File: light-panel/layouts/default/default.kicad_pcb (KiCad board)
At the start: 2 copper layers, 150 x 29.7 mm, 70 parts

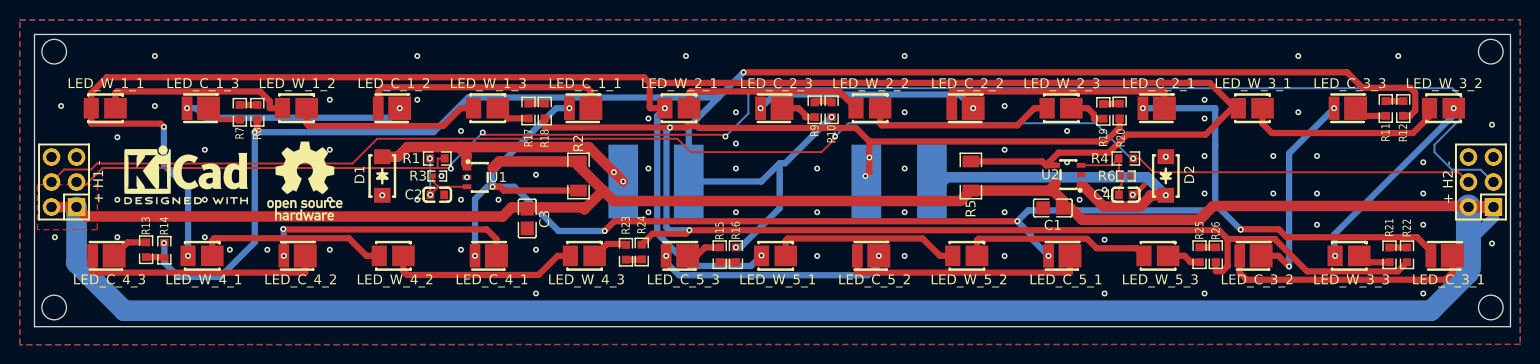
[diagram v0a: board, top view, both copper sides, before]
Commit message: panel router
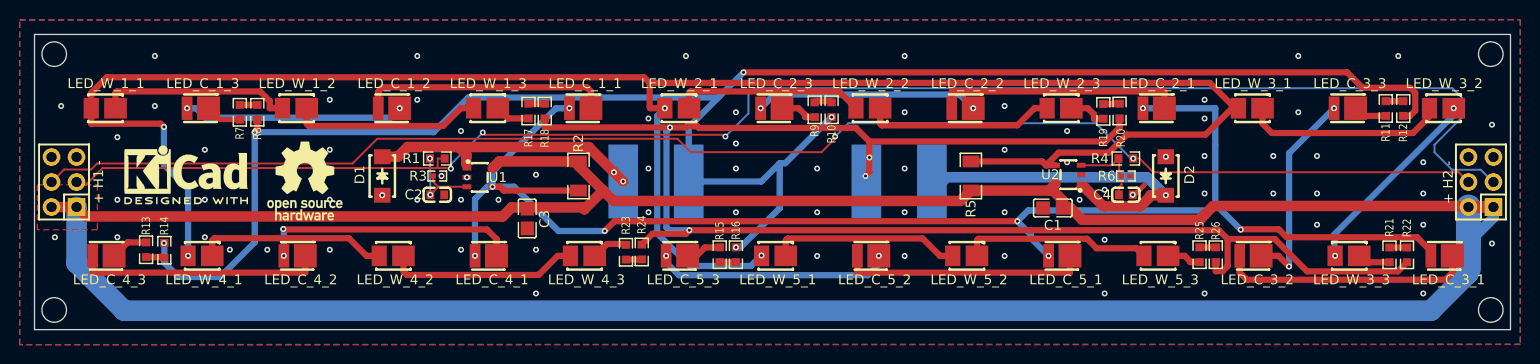
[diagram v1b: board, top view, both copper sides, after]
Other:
- board size 150 x 29.7 mm -> 150 x 30 mm
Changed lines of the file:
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@@
 	)
 	(gr_circle
-		(center 52 99.25)
-		(end 53.25 99.25)
+		(center 52 99.5)
+		(end 53.25 99.5)
 		(stroke
 			(width 0.05)
@@
 	)
 	(gr_circle
-		(center 198 99.25)
-		(end 199.25 99.25)
+		(center 198 99.5)
+		(end 199.25 99.5)
 		(stroke
 			(width 0.05)
@@
 	)
 	(gr_circle
-		(center 198 125.25)
-		(end 199.25 125.25)
+		(center 198 125.5)
+		(end 199.25 125.5)
 		(stroke
 			(width 0.05)
@@
 	(gr_rect
 		(start 50 97.5)
-		(end 200 127.2)
+		(end 200 127.5)
 		(stroke
 			(width 0.05)
@@
 	)
 	(gr_circle
-		(center 52 125.25)
-		(end 53.25 125.25)
+		(center 52 125.5)
+		(end 53.25 125.5)
 		(stroke
 			(width 0.05)
